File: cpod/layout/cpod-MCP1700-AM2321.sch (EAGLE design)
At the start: 14 parts, among them IC1 PCF8563DIP, Y1 32.768kHz

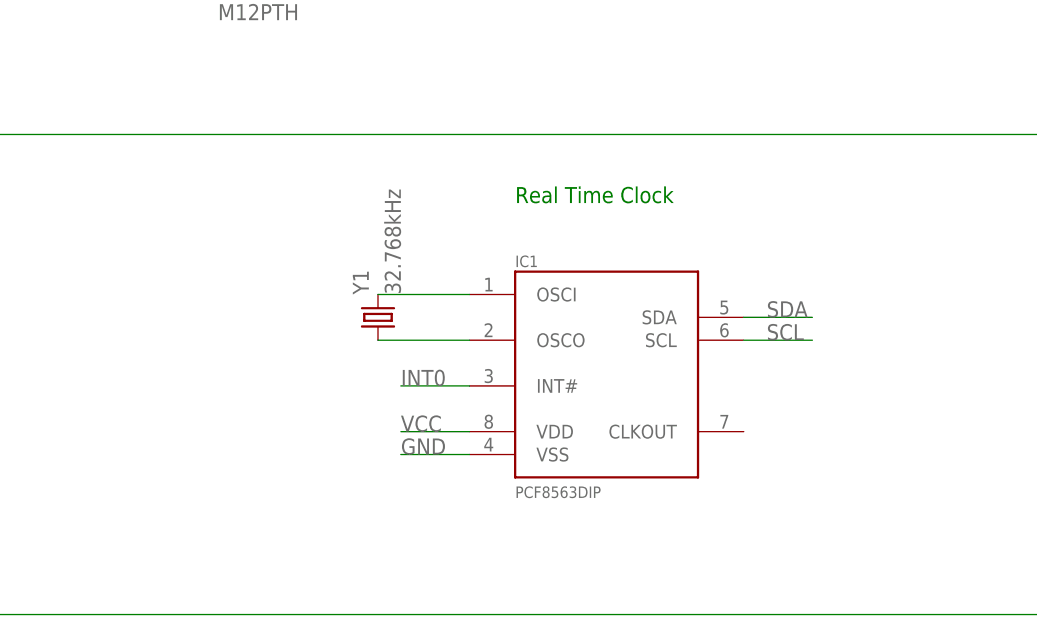
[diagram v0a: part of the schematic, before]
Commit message: 上拉电阻布线
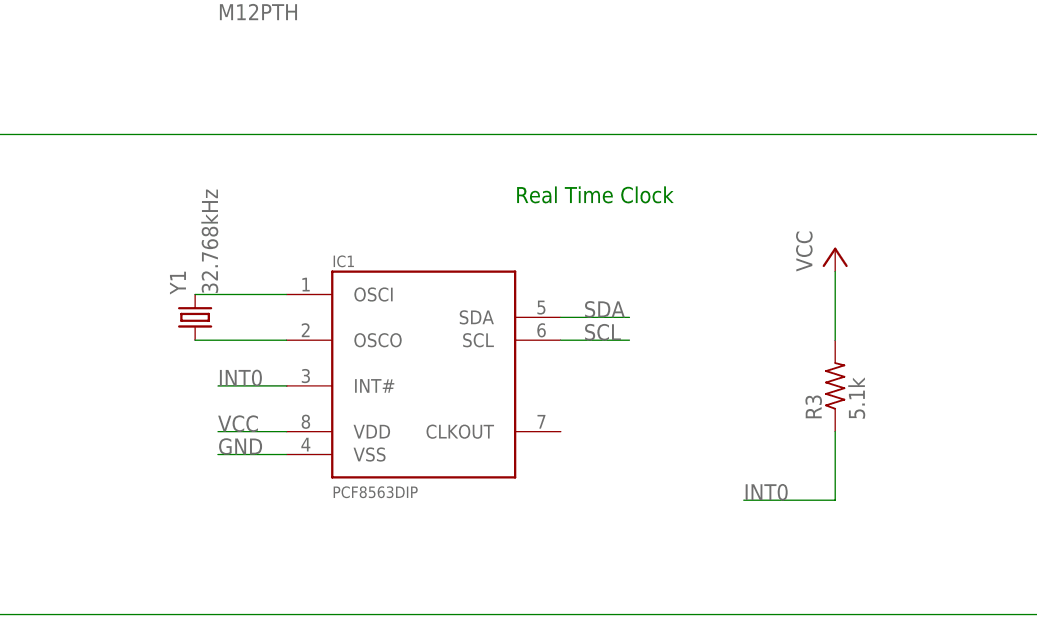
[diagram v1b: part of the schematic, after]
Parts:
- added R3: 5.1k, rcl:R-US_0204/7
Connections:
- net INT0: now also R3.1
- net VCC: now also R3.2
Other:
- moved on the sheet: IC1, Y1
